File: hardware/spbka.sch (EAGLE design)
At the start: 20 parts, among them Q1 DMP1045U-7, U1 ATTINY10, U2 LM4041DYM3-1.2, U3 MCP6L01T

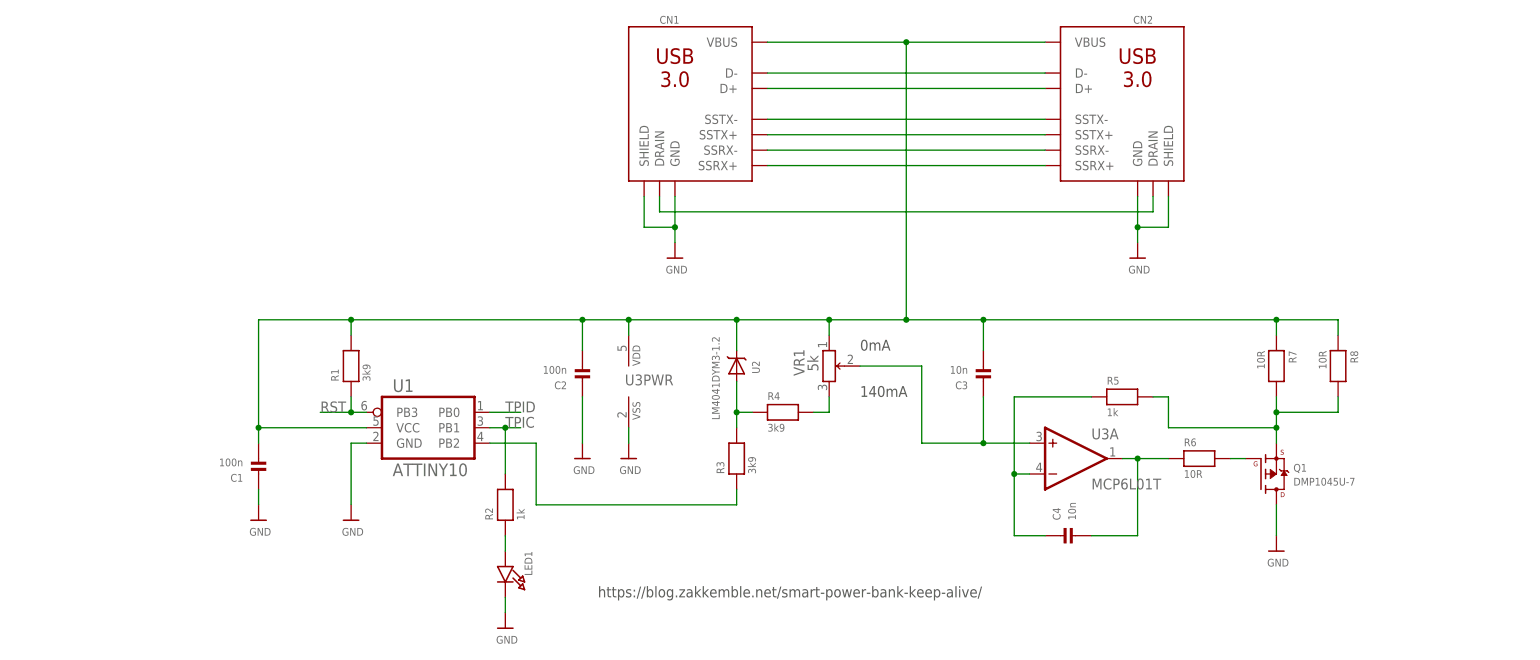
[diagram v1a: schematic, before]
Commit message: hardware v2.1
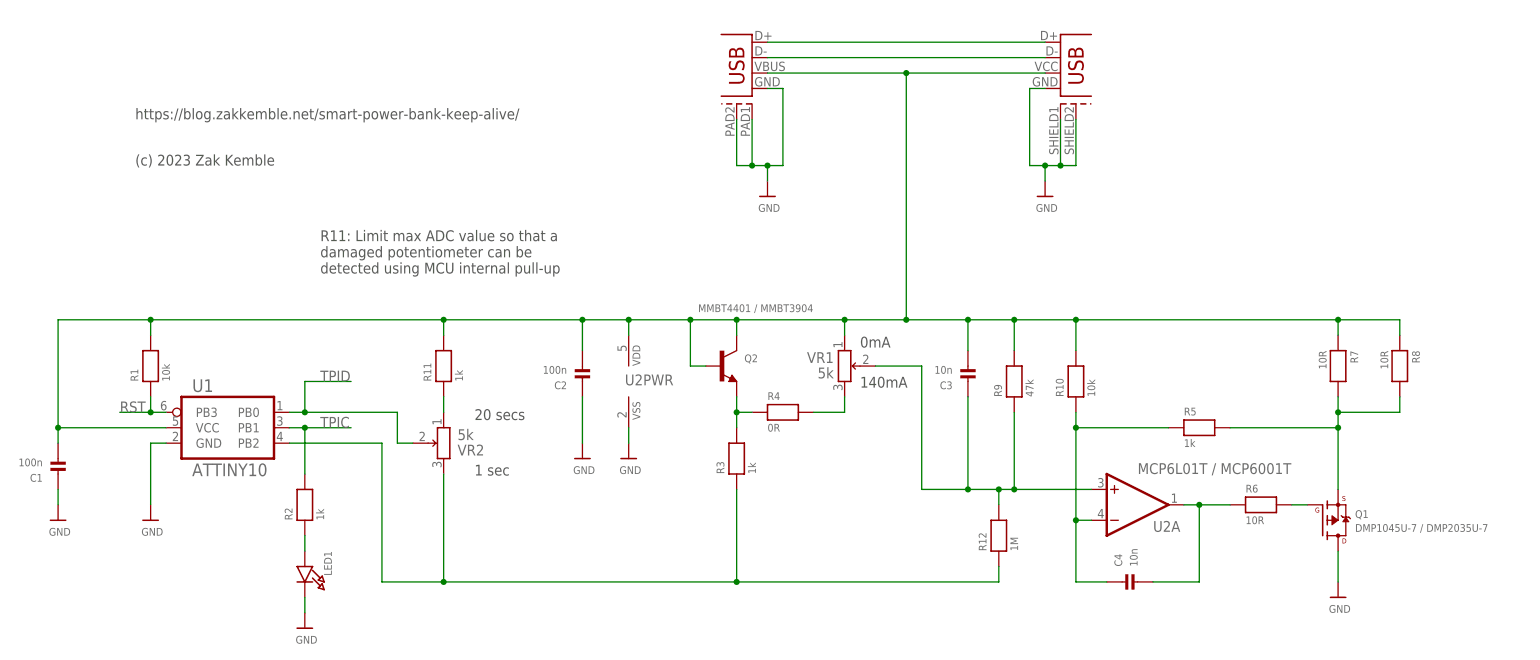
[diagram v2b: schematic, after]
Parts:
- removed CN1: (no value), zak:USB-3TYPE-A-SMD-PLUG-SLOT
- removed CN2: (no value), zak:USB-3TYPE-A-SMD-SOCKET-SLOT
- removed U3: MCP6L01T, zak:OPAMP_SINGLECONFIG1_SMPAD
- added Q2: MMBT4401 / MMBT3904, microbuilder:TRANSISTOR_NPN
- added R10: 10k, zak:RESISTOR0402_XSMALL
- added R11: 1k, zak:RESISTOR0402_XSMALL
- added R12: 1M, zak:RESISTOR0402_XSMALL
- added R9: 47k, zak:RESISTOR0402_XSMALL
- added USB1: USB-TYPE-AHORZ, zak:USB-TYPE-AHORZ
- added USB2: (no value), zak:USB-PLUG
- added VR2: 5k, zak:POTENTIOMETERBOURNS3MM
- C1, C2, C3, C4: device zak:CAP_CERAMIC0402_SMALL -> zak:CAP_CERAMIC0402_XSMALL
- Q1: value DMP1045U-7 -> DMP1045U-7 / DMP2035U-7
- R1: value 3k9 -> 10k; device zak:RESISTOR0402_SMALL -> zak:RESISTOR0402_XSMALL
- R2, R5, R6, R7, R8: device zak:RESISTOR0402_SMALL -> zak:RESISTOR0402_XSMALL
- R3: value 3k9 -> 1k; device zak:RESISTOR0402_SMALL -> zak:RESISTOR0402_XSMALL
- R4: value 3k9 -> 0R; device zak:RESISTOR0402_SMALL -> zak:RESISTOR0402_XSMALL
- U2: value LM4041DYM3-1.2 -> MCP6L01T / MCP6001T; device zak:DIODE-ZENERSOT-23-SLIM -> zak:OPAMP_SINGLECONFIG1_SMPAD
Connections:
- removed net N$13: R3.1, U1.PB2
- removed net N$14: CN1.SSTX-, CN2.SSTX-
- removed net N$15: CN1.D+, CN2.D+
- removed net N$16: CN1.D-, CN2.D-
- removed net N$19: C1.P$2, C2.P$2, C3.P$2, CN1.VBUS, CN2.VBUS, R1.2, R7.1, R8.1, U1.VCC, U2.C, U3PWR.VDD, VR1.1A
- removed net N$9 (its old number): CN1.SSRX-, CN2.SSRX-
- new net N$1: Q2.E, R3.2, R4.1
- new net VBUS: C1.P$2, C2.P$2, C3.P$2, Q2.B, Q2.C, R1.2, R10.2, R11.2, R7.1, R8.1, R9.2, U1.VCC, U2PWR.VDD, USB1.VBUS, USB2.VBUS, VR1.1A
- net GND: now also U2PWR.VSS, USB1.GND, USB1.SHEILD1, USB1.SHEILD2, USB2.GND, USB2.SHEILD1, USB2.SHEILD2; no longer CN1.GND, CN1.SHIELD, CN2.GND, CN2.SHIELD, U3PWR.VSS
- net N$11: now also R12.2, R9.1, U2A.+IN; no longer U3A.+IN
- net N$12: now also R11.1, VR2.1A; no longer CN1.SSTX+, CN2.SSTX+
- net N$3: now also U2A.OUT; no longer U3A.OUT
- net N$5: now also USB1.D+, USB2.D+; no longer CN1.DRAIN, CN2.DRAIN
- net N$6: now also USB1.D-, USB2.D-; no longer CN1.SSRX+, CN2.SSRX+
- net N$7: now also R12.1, R3.1, U1.PB2, VR2.1E; no longer R3.2, R4.1, U2.A
- net N$8: now also R10.1, U2A.-IN; no longer U3A.-IN
- net TPID: now also VR2.1S
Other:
- note added: "(c) 2023 Zak Kemble"
- note added: "1 sec"
- note added: "20 secs"
- note added: "R11: Limit max ADC value so that a damaged potentiometer can be detected using MCU internal pull-up"
- moved on the sheet: C1, C3, C4, LED1, Q1, R1, R2, R5, R6, R7, R8, U1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
